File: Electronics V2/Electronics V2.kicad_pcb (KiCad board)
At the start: 2 copper layers, 102 x 62 mm, 88 parts, among them J1 MOT_L, J2 MOT_R, J3 SD_Card, J4 USB_C_Receptacle_USB2.0_14P, J5 Power Probes, J6 L1, J7 L2, Q1 BC547, SW1 BTN_0, SW2 MSTP_SEL, SW3 RST, SW4 BOOT, SW5 BTN_1, SW6 BTN_2, SW7 BTN_3, SW8 INCR_0, U1 NCP1117-3.3_SOT223, U10 TVS1400DRV, U11 TVS1400DRV, U2 TMC2209, U3 ESP32-S3-WROOM-1, U4 DAC081C081CIMK, U5 IMU_L, U6 IMU_R, U7 NCP1117-3.3_SOT223, U8 SSD1036, U9 TMC2209

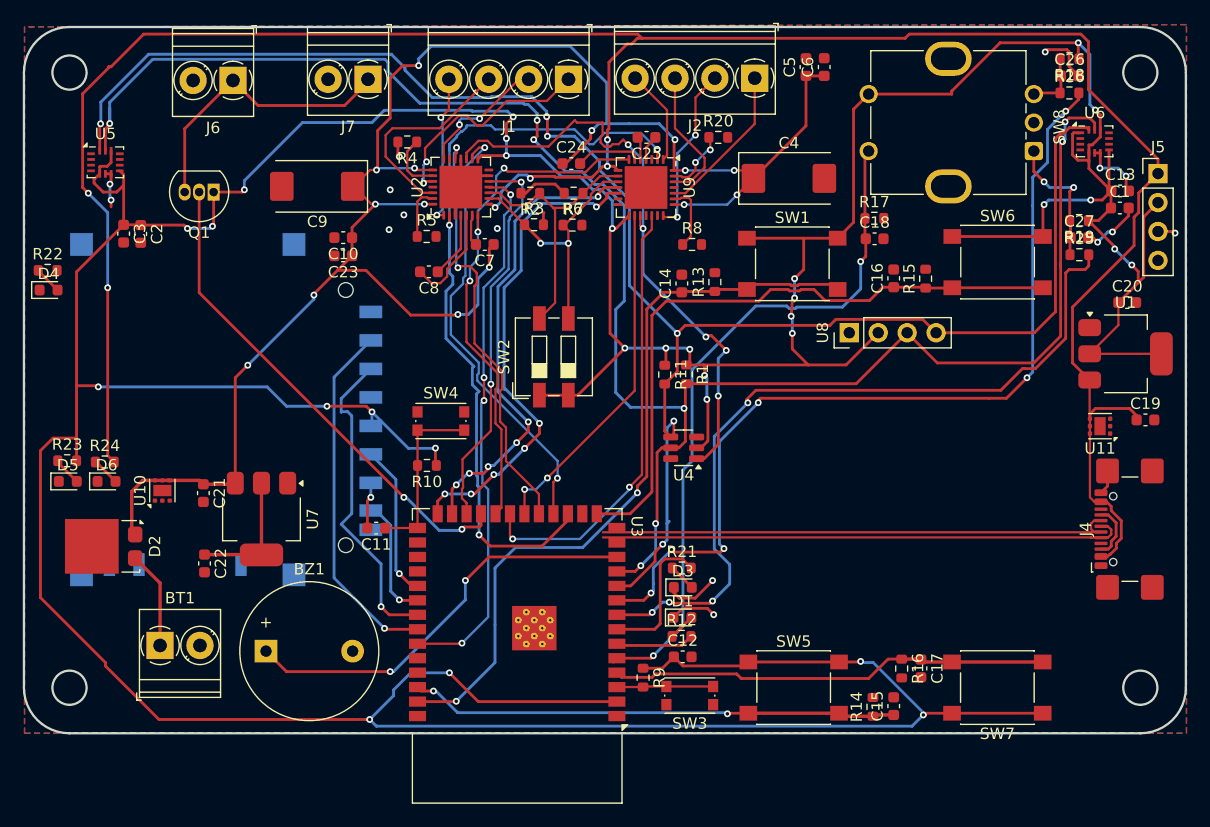
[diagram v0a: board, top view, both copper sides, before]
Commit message: completed pcb fr this time
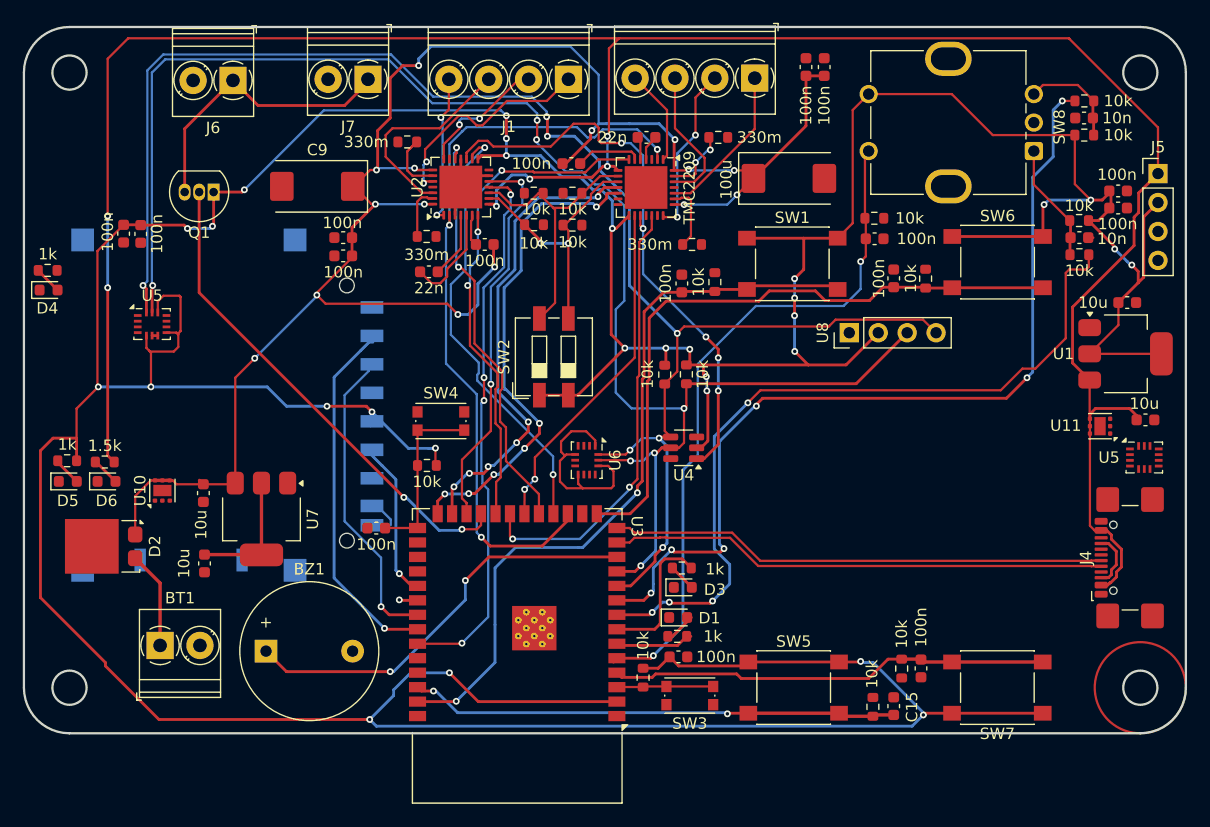
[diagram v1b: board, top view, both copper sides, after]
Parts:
- removed the U5 at (108.6, 78.3)
- added U5: IMU_L, Package_LGA:Bosch_LGA-14_3x2.5mm_P0.5mm, F.Cu at (112.7, 92.5)
- added U5: IMU_L, Package_LGA:Bosch_LGA-14_3x2.5mm_P0.5mm, F.Cu at (199.8, 104.2)
- moved U6 52.6 mm to (150.8, 104.4), turned to -90 degrees
- moved 10k 6.82 mm to (194.5, 75.9), turned to 0 degrees
- moved 10n 3.91 mm to (194.5, 74.4), turned to 180 degrees
- moved J4 2.51 mm to (199.7, 113.0)
- moved 10k 1.49 mm to (194.5, 72.9), turned to 180 degrees
- moved J3 0.41 mm to (117.0, 99.6)
- moved 100n 0.38 mm to (158.9, 121.7)
- moved 1k 0.38 mm to (158.8, 119.9)
- moved D1 0.38 mm to (158.9, 118.2)
- moved 10k 0.30 mm to (146.2, 81.0)
- moved 100n 0.18 mm to (197.5, 80.8)
- moved 100n 0.15 mm to (197.5, 82.3)
- moved 10k 0.10 mm to (149.6, 81.0)
- renumbered R24 to 1.5k, C3 to 100n, C11 to 100n, C24 to 100n, C6 to 100n, C17 to 100n, C14 to 100n, C13 to 100n, C5 to 100n, C16 to 100n, C12 to 100n, C7 to 100n, C1 to 100n, C18 to 100n, C10 to 100n, C23 to 100n, C2 to 100n, C4 to 100u, R2 to 10k, R19 to 10k, R1 to 10k, R15 to 10k, R14 to 10k, R9 to 10k, R11 to 10k, R6 to 10k, R16 to 10k, R26 to 10k, R18 to 10k, R25 to 10k, R17 to 10k, R13 to 10k, R7 to 10k, R3 to 10k, R10 to 10k, C26 to 10n, C27 to 10n, C22 to 10u, C19 to 10u, C21 to 10u, C20 to 10u, R23 to 1k, R12 to 1k, R21 to 1k, R22 to 1k, C8 to 22n, C25 to 22n, R8 to 330m, R4 to 330m, R20 to 330m, R5 to 330m, U9 to TMC2209
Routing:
- net GND: track 51.3 -> 9.29 mm, vias 16 -> 0
- net /SCL: track 163.6 -> 140.9 mm, vias 8 -> 7
- net /SDA: track 155.4 -> 141.2 mm, vias 6 -> 7
- net /MISO: track 10.8 -> 4.26 mm
- net Net-(C26-Pad1): track 5.40 -> 9.37 mm
- net /D+: track 46.2 -> 43.7 mm
- net /D-: track 46.2 -> 43.7 mm
- net /VREF: track 53.3 -> 51.3 mm
- net Net-(C27-Pad1): track 12.0 -> 10.5 mm, vias 2 -> 0
- net /CS_SD: track 31.4 -> 32.8 mm
- net +5V: track 211.1 -> 209.9 mm
- net /SCLK: track 13.6 -> 14.7 mm
- net /~{EN}: track 68.5 -> 67.5 mm
- net /MOSI: track 28.0 -> 27.1 mm
- net /DIR_L: track 37.5 -> 36.6 mm
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- removed copper zone on B.Cu, net GND
- removed copper zone on F.Cu, net GND
